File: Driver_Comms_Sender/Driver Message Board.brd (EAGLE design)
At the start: 160 x 100 mm, 14 parts, among them U1 XBEE_PRO_S3B

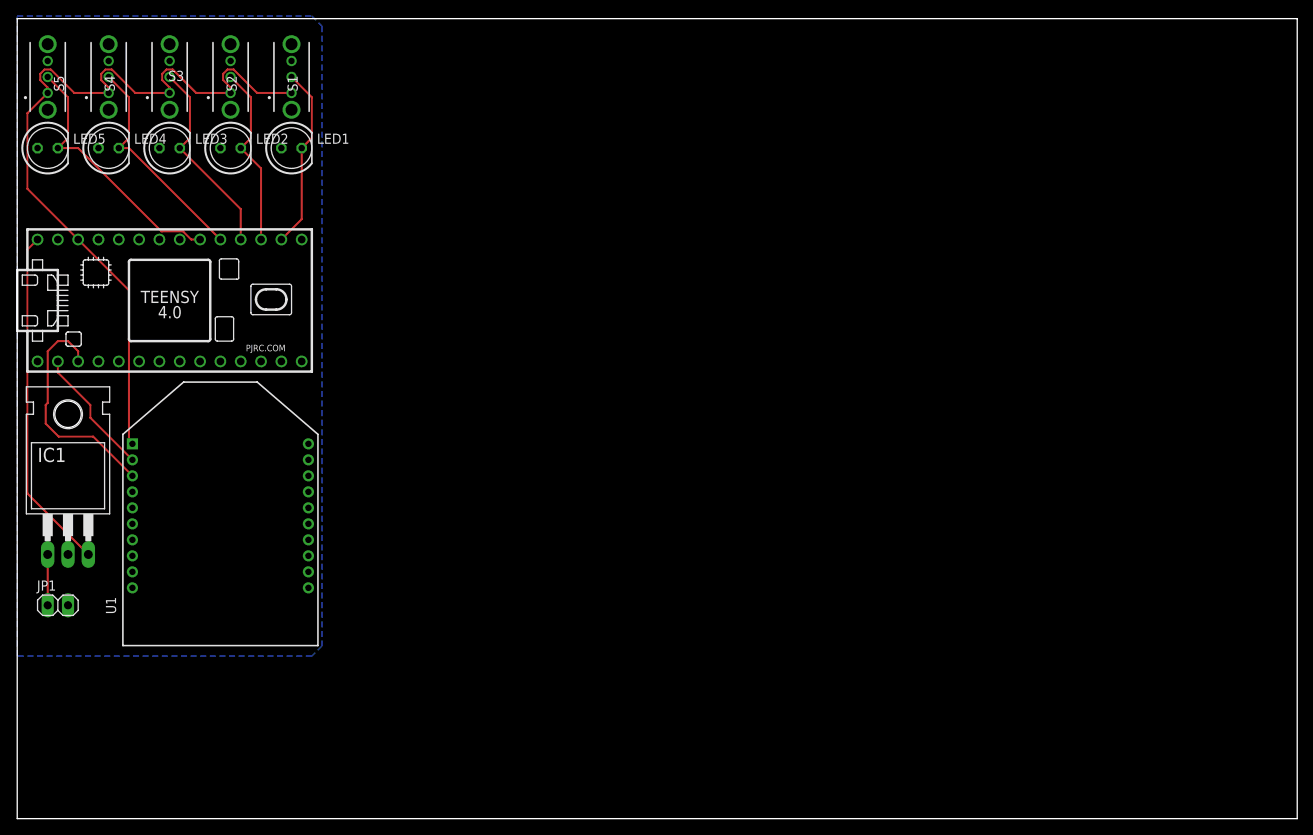
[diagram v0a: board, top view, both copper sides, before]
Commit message: Finalized PCB and started code
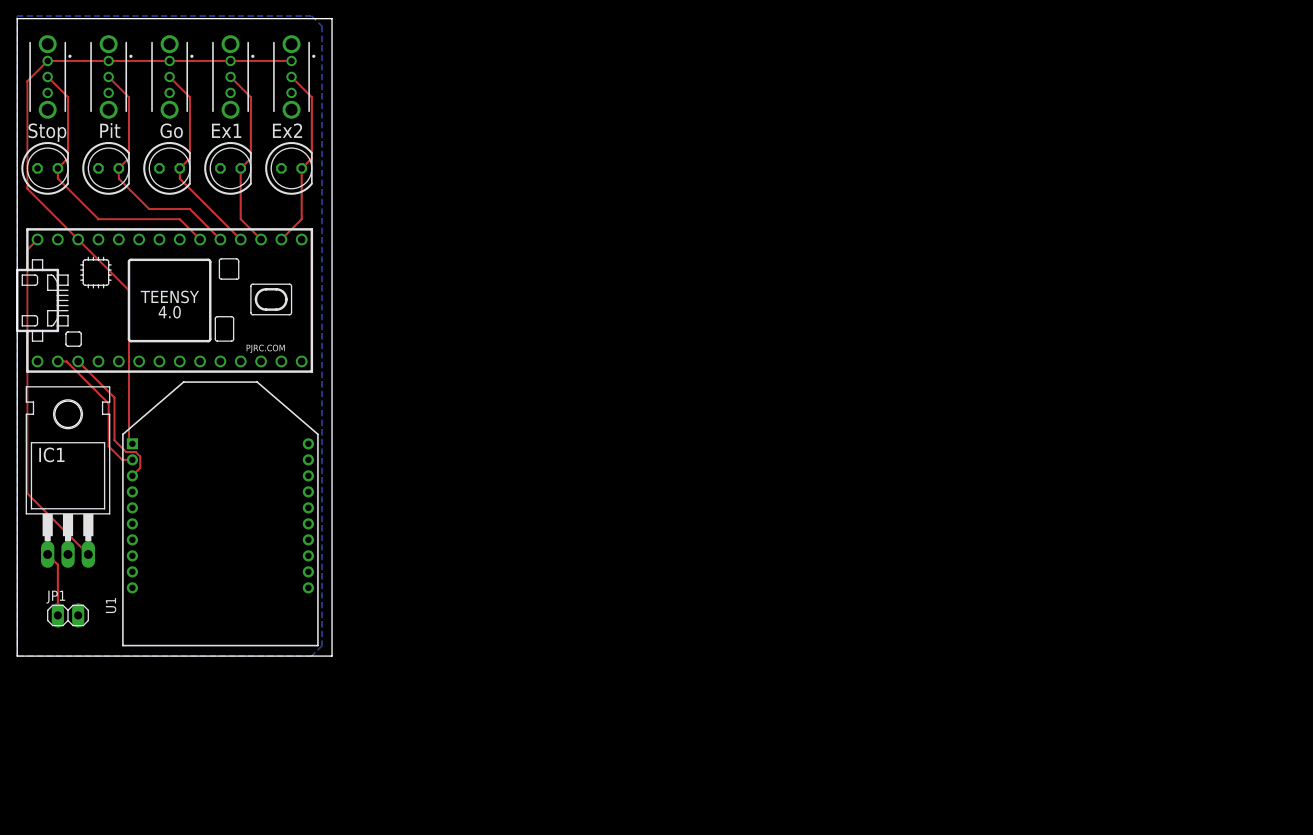
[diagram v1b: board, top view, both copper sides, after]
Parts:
- moved LED1 2.54 mm to (34.3, 81.3)
- moved LED2 2.54 mm to (26.7, 81.3)
- moved LED3 2.54 mm to (19.1, 81.3)
- moved LED4 2.54 mm to (11.4, 81.3)
- moved LED5 2.54 mm to (3.81, 81.3)
- moved JP1 1.80 mm to (6.35, 25.4)
- turned S1 to 270 degrees
- turned S2 to 270 degrees
- turned S3 to 270 degrees
- turned S4 to 270 degrees
- turned S5 to 270 degrees
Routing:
- net 3V_TEENSY: track 103.0 -> 84.8 mm
- net XBEE_RX: track 28.8 -> 18.6 mm
- net A4: track 33.0 -> 35.2 mm
- net A3: track 27.9 -> 30.1 mm
- net VCC: track 6.35 -> 8.15 mm
- net XBEE_TX: track 16.2 -> 17.6 mm
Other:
- board size 160 x 100 mm -> 39.4 x 79.7 mm
- board text added: "Ex1"
- board text added: "Ex2"
- board text added: "Go"
- board text added: "Pit"
- board text added: "Stop"
